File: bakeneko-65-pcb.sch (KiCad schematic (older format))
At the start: 160 parts, among them J1 JST SH 4-pin, J2 AVR-ISP-6, SW1 Reset, U1 USBLC6-2SC6, U2 ATmega32U4-AU, Y1 16MHz

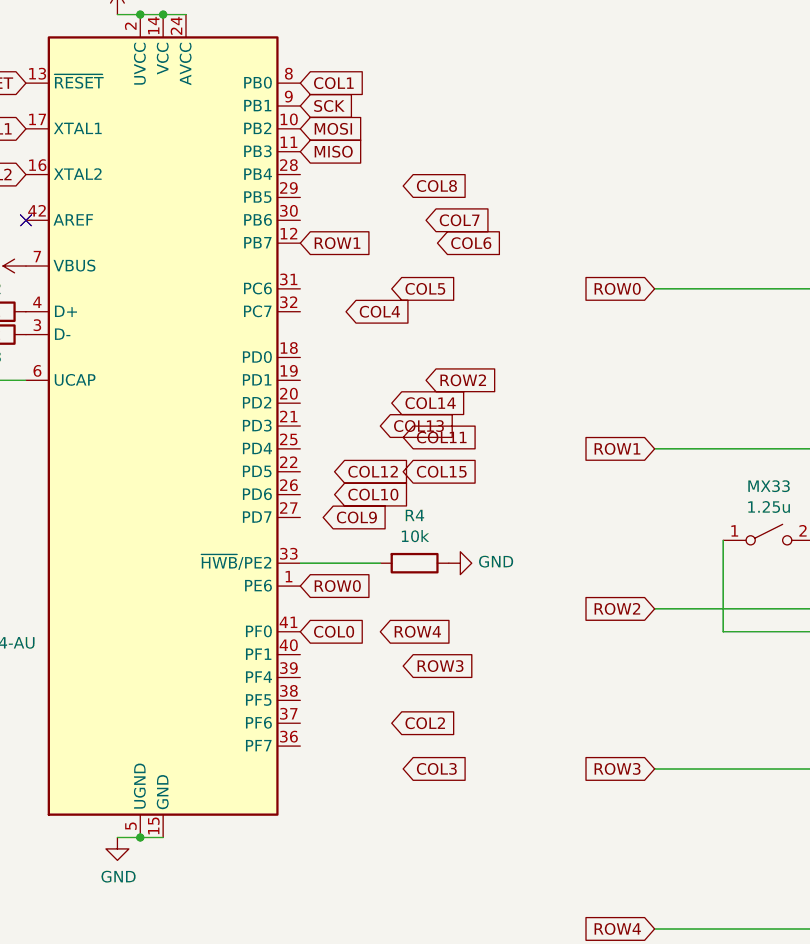
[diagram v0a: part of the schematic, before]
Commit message: Update PCB
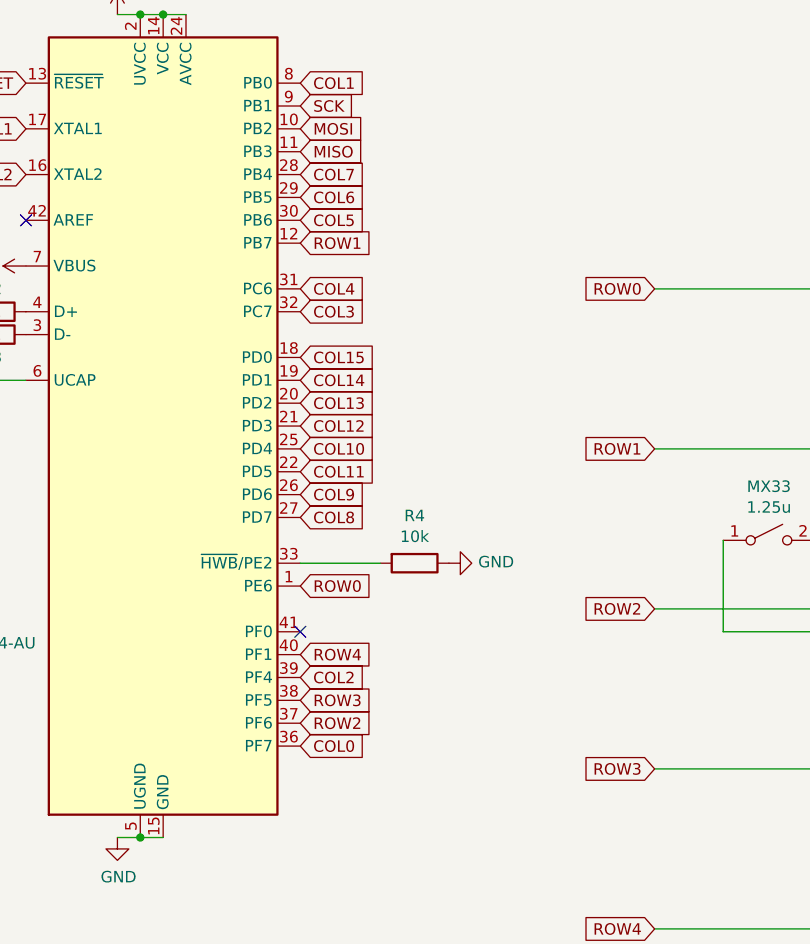
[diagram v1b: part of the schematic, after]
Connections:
- net COL0: now also U2.36 (PF7); no longer U2.41 (PF0)
- net COL10: now also U2.25 (PD4)
- net COL11: now also U2.22 (PD5)
- net COL12: now also U2.21 (PD3)
- net COL13: now also U2.20 (PD2)
- net COL14: now also U2.19 (PD1)
- net COL15: now also U2.18 (PD0)
- net COL2: now also U2.39 (PF4)
- net COL3: now also U2.32 (PC7)
- net COL4: now also U2.31 (PC6)
- net COL5: now also U2.30 (PB6)
- net COL6: now also U2.29 (PB5)
- net COL7: now also U2.28 (PB4)
- net COL8: now also U2.27 (PD7)
- net COL9: now also U2.26 (PD6)
- net ROW2: now also U2.37 (PF6)
- net ROW3: now also U2.38 (PF5)
- net ROW4: now also U2.40 (PF1)
- no-connect marks 1 -> 2
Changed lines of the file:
@@
-$EndComp
-$Comp
-L Switch:SW_SPST MX5
-U 1 1 5F2C356D
-P 9050 6050
-F 0 "MX5" H 9050 6285 50  0000 C CNN
-F 1 "1u" H 9050 6194 50  0000 C CNN
-F 2 "Button_Switch_Keyboard:SW_Cherry_MX_1.00u_PCB" H 9050 6050 50  0001 C CNN
-F 3 "~" H 9050 6050 50  0001 C CNN
-	1    9050 6050
-	1    0    0    -1
 $EndComp
 $Comp
@@
 Text GLabel 6650 5450 2    50   Input ~ 0
 COL0
-Text GLabel 4700 7150 2    50   Input ~ 0
+Text GLabel 4250 6650 2    50   Input ~ 0
 COL15
-Text GLabel 4650 6850 2    50   Input ~ 0
+Text GLabel 4250 6750 2    50   Input ~ 0
 COL14
-Text GLabel 4600 6950 2    50   Input ~ 0
+Text GLabel 4250 6850 2    50   Input ~ 0
 COL13
-Text GLabel 4400 7150 2    50   Input ~ 0
+Text GLabel 4250 6950 2    50   Input ~ 0
 COL12
-Text GLabel 4700 7000 2    50   Input ~ 0
+Text GLabel 4250 7150 2    50   Input ~ 0
 COL11
-Text GLabel 4400 7250 2    50   Input ~ 0
+Text GLabel 4250 7050 2    50   Input ~ 0
 COL10
-Text GLabel 4350 7350 2    50   Input ~ 0
+Text GLabel 4250 7250 2    50   Input ~ 0
 COL9
-Text GLabel 4700 5900 2    50   Input ~ 0
+Text GLabel 4250 7350 2    50   Input ~ 0
 COL8
-Text GLabel 4800 6050 2    50   Input ~ 0
+Text GLabel 4250 5850 2    50   Input ~ 0
 COL7
-Text GLabel 4850 6150 2    50   Input ~ 0
+Text GLabel 4250 5950 2    50   Input ~ 0
 COL6
-Text GLabel 4650 6350 2    50   Input ~ 0
+Text GLabel 4250 6050 2    50   Input ~ 0
 COL5
-Text GLabel 4450 6450 2    50   Input ~ 0
+Text GLabel 4250 6350 2    50   Input ~ 0
 COL4
-Text GLabel 4700 8450 2    50   Input ~ 0
-COL3
-Text GLabel 4650 8250 2    50   Input ~ 0
+Text GLabel 4250 8050 2    50   Input ~ 0
 COL2
 Text GLabel 4250 5450 2    50   Input ~ 0
 COL1
-Text GLabel 4250 7850 2    50   Input ~ 0
+Text GLabel 4250 8350 2    50   Input ~ 0
 COL0
 Text GLabel 4250 6150 2    50   Input ~ 0
 ROW1
-Text GLabel 4800 6750 2    50   Input ~ 0
+Text GLabel 4250 8250 2    50   Input ~ 0
 ROW2
-Text GLabel 4700 8000 2    50   Input ~ 0
+Text GLabel 4250 8150 2    50   Input ~ 0
 ROW3
-Text GLabel 4600 7850 2    50   Input ~ 0
+Text GLabel 4250 7950 2    50   Input ~ 0
 ROW4
 Wire Wire Line
@@
 	6300 2050 6300 1900
 Connection ~ 5900 2050
+$Comp
+L Switch:SW_SPST MX5
+U 1 1 5F2C356D
+P 9050 6050
+F 0 "MX5" H 9050 6285 50  0000 C CNN
+F 1 "1u" H 9050 6194 50  0000 C CNN
+F 2 "Button_Switch_Keyboard:SW_Cherry_MX_1.00u_PCB" H 9050 6050 50  0001 C CNN
+F 3 "~" H 9050 6050 50  0001 C CNN
+	1    9050 6050
+	1    0    0    -1
+$EndComp
+Text GLabel 4250 6450 2    50   Input ~ 0
+COL3
+NoConn ~ 4250 7850
 $EndSCHEMATC
